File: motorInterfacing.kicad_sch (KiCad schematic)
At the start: 6 parts, among them J1 Conn_01x02, J2 Conn_01x02, J3 Conn_01x01, J4 Conn_01x01

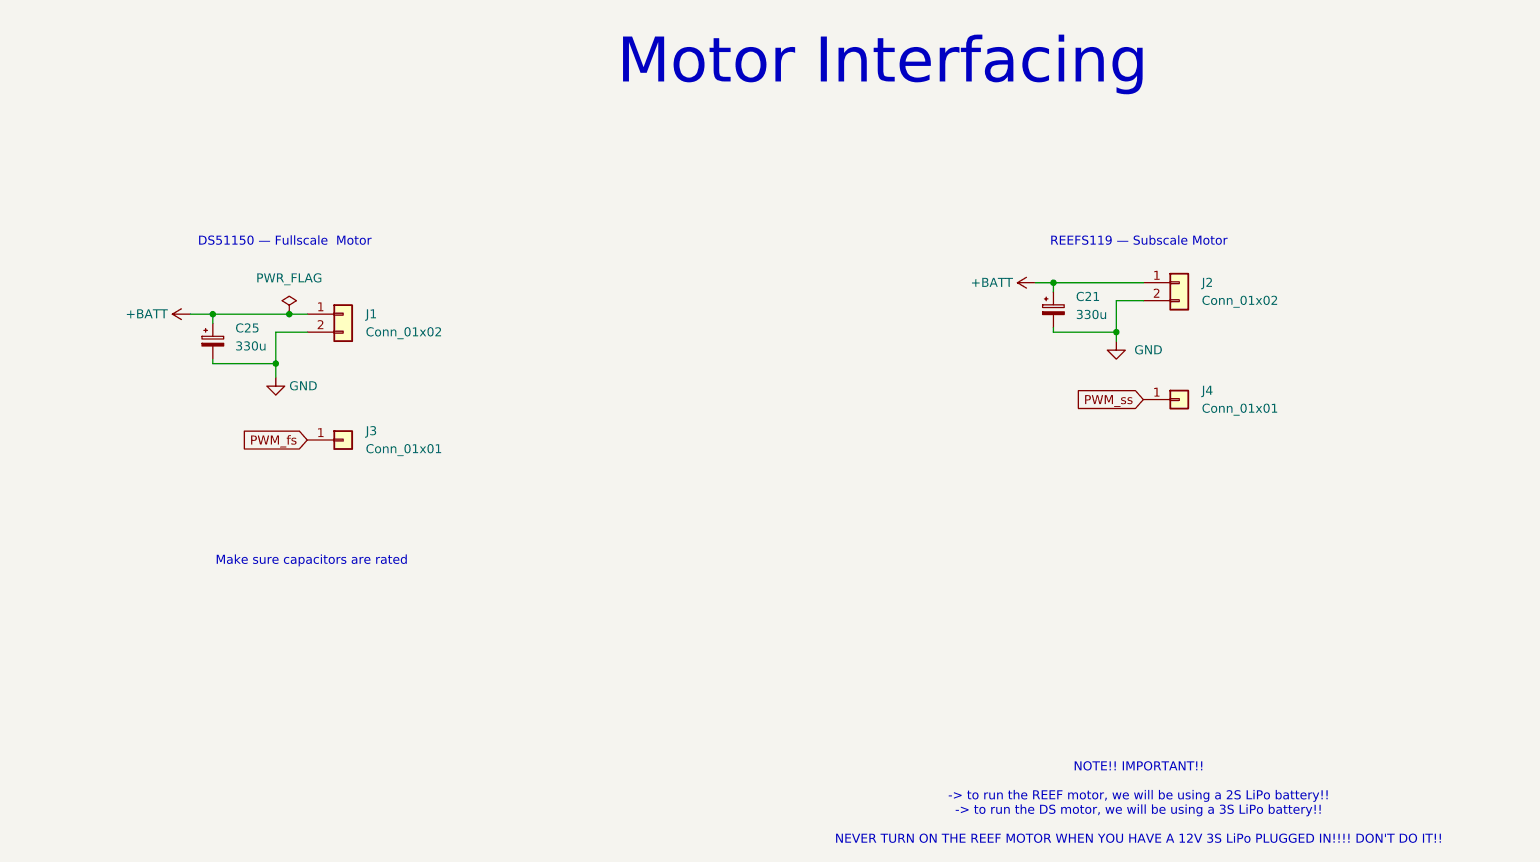
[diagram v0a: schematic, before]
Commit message: created PCB and layout
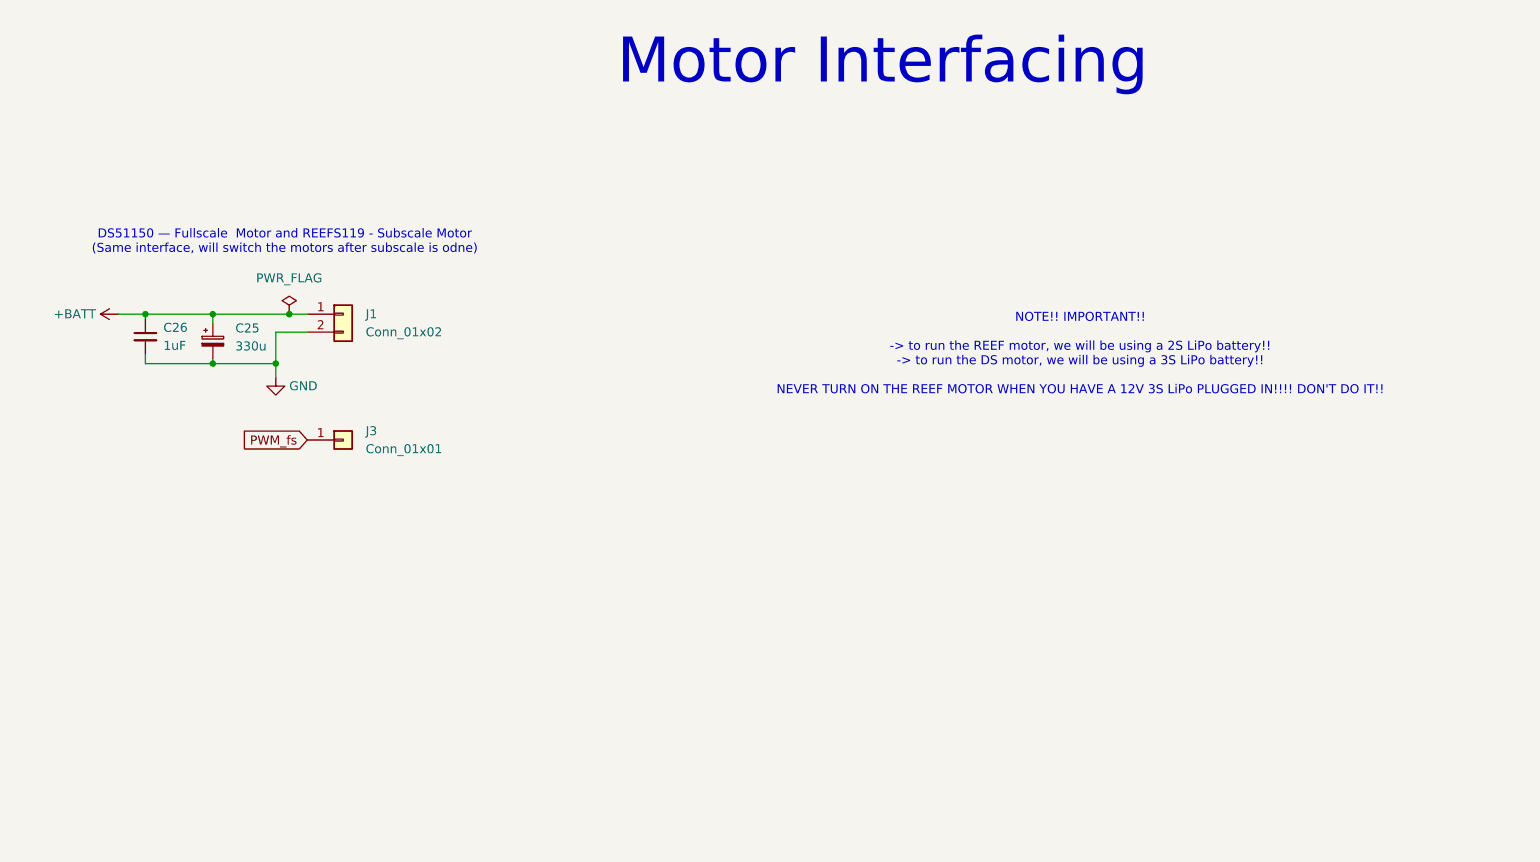
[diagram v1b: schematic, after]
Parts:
- removed C21: 330u, Capacitor_SMD:C_0603_1608Metric, symbol Device:C_Polarized_Small
- removed J2: Conn_01x02, symbol Connector_Generic:Conn_01x02
- removed J4: Conn_01x01, symbol Connector_Generic:Conn_01x01
- added C26: 1uF, Capacitor_SMD:C_0603_1608Metric, symbol Device:C_Small
- J1: footprint (none) -> Connector_AMASS:AMASS_XT30U-F_1x02_P5.0mm_Vertical
- J3: footprint (none) -> Connector_Wire:SolderWire-0.5sqmm_1x01_D0.9mm_OD2.1mm
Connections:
- net +BATT: now also C26.1
- net GND: now also C26.2
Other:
- note added: "DS51150 — Fullscale Motor and REEFS119 - Subscale Motor (Same interface, will switch the motors after subscale is odne)"
- note removed: "DS51150 — Fullscale Motor"
- note removed: "Make sure capacitors are rated"
- note removed: "REEFS119 — Subscale Motor"
